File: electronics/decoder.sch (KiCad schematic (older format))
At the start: 8 parts, among them U33 AT28C64B, U40 AT28C64B, U41 AT28C64B, U44 AT28C64B

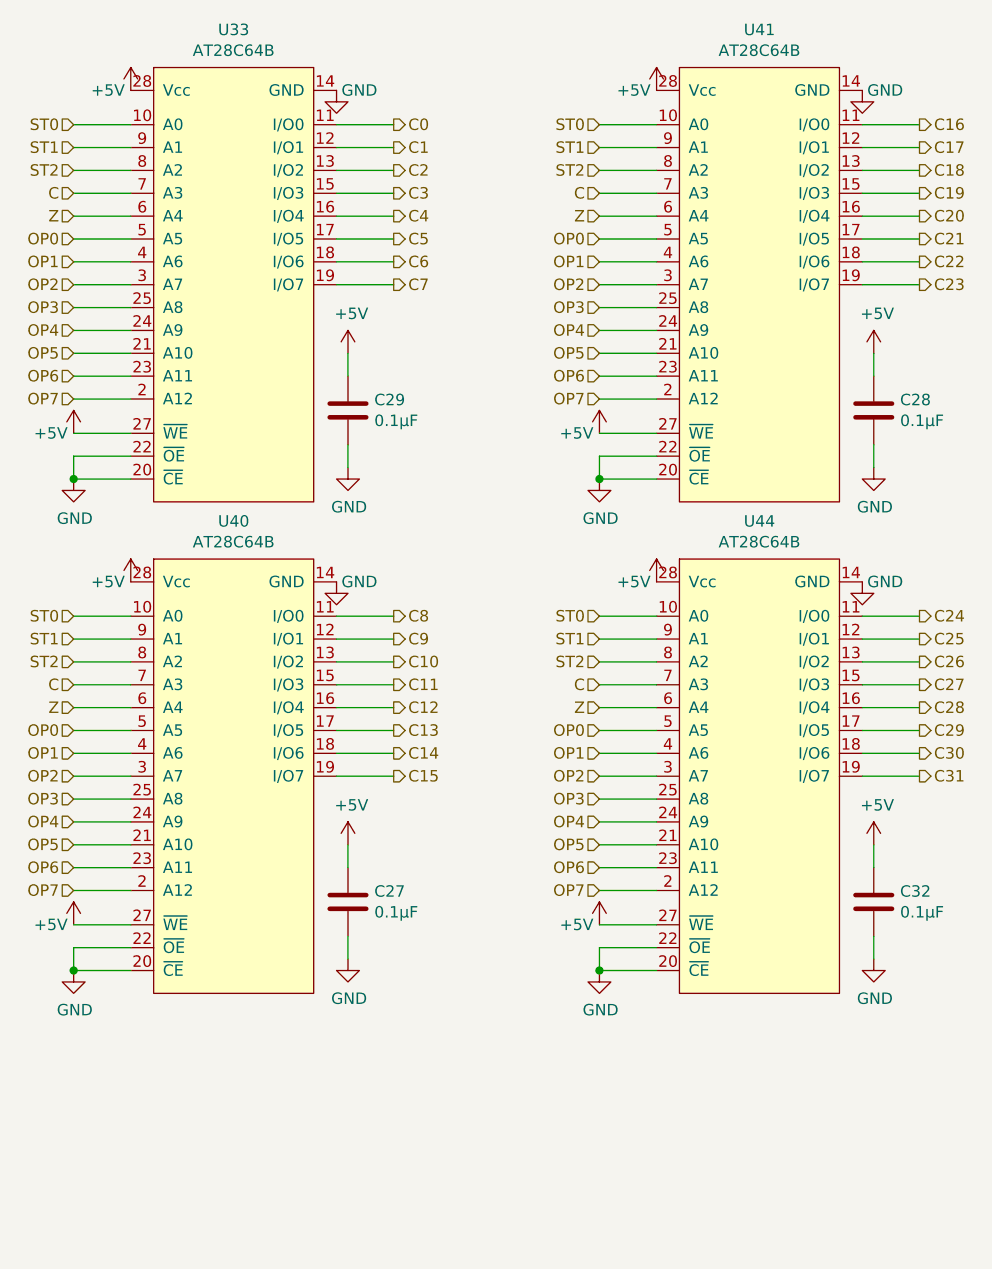
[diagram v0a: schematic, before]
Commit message: Some initial electronics design
Not everything done yet, just committing to show progress and to get the changes out of the way.
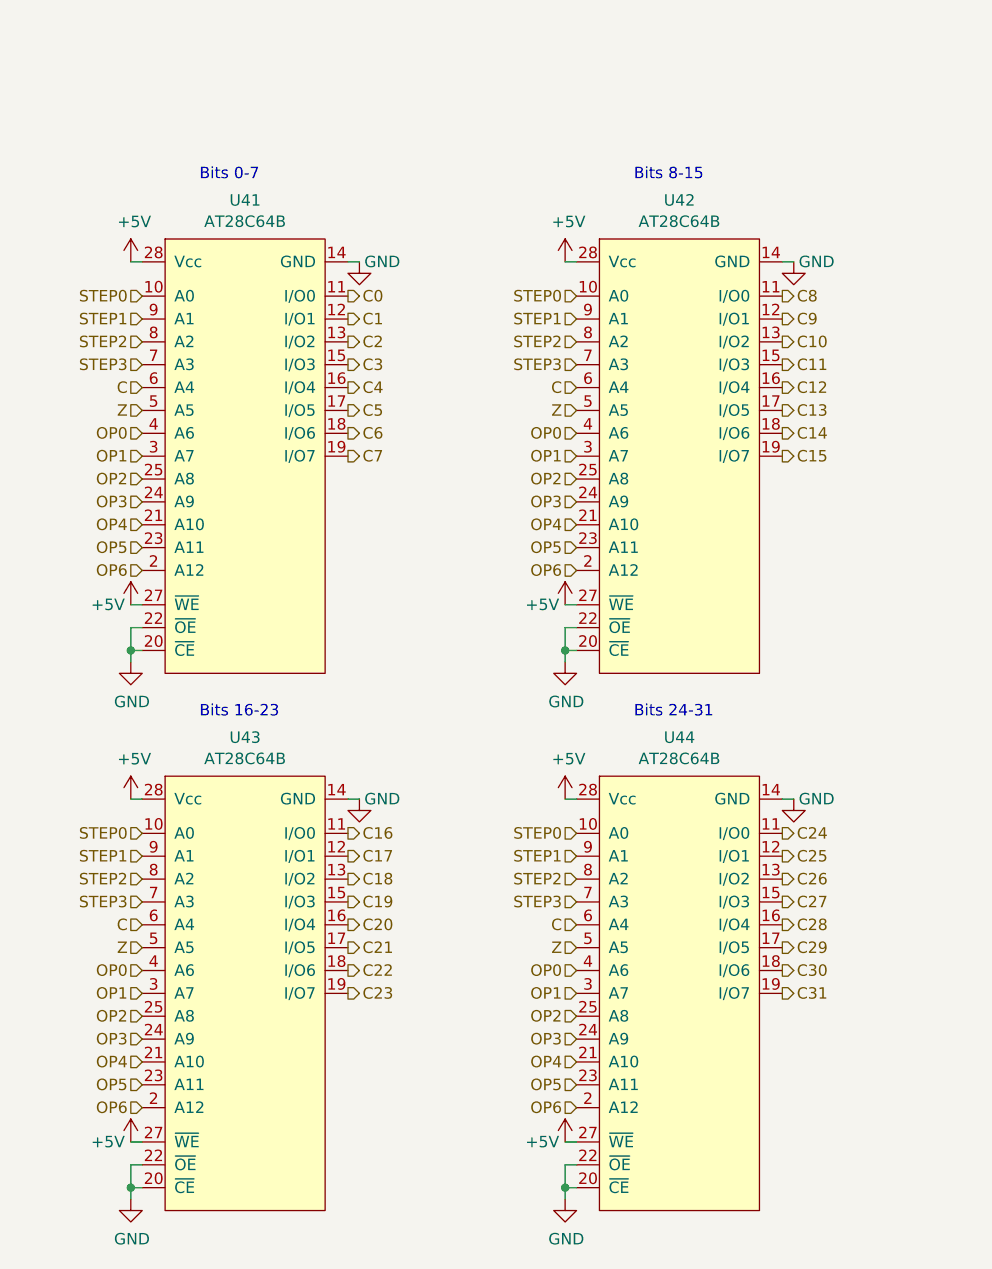
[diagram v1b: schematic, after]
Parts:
- removed C27, C28, C29, C32: 0.1µF, Capacitor_THT:CP_Radial_D4.0mm_P1.50mm, symbol Device:C
- removed U33, U40: AT28C64B, Package_DIP:AT28C64B, symbol misc_components:AT28C64B
- added U42, U43: AT28C64B, symbol misc_components:AT28C64B
- U41, U44: footprint Package_DIP:AT28C64B -> (none)
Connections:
- net OP7 is gone; now on net OP6: U41.2 (A12), U44.2 (A12)
- net +5V: now also U42.27 (~WE), U42.28 (Vcc), U43.27 (~WE), U43.28 (Vcc)
- net C: now also U41.6 (A4), U44.6 (A4), U42.6 (A4), U43.6 (A4); no longer U41.7 (A3), U44.7 (A3)
- net C0: now also U41.11 (I/O0)
- net C1: now also U41.12 (I/O1)
- net C10: now also U42.13 (I/O2)
- net C11: now also U42.15 (I/O3)
- net C12: now also U42.16 (I/O4)
- net C13: now also U42.17 (I/O5)
- net C14: now also U42.18 (I/O6)
- net C15: now also U42.19 (I/O7)
- net C16: now also U43.11 (I/O0); no longer U41.11 (I/O0)
- net C17: now also U43.12 (I/O1); no longer U41.12 (I/O1)
- net C18: now also U43.13 (I/O2); no longer U41.13 (I/O2)
- net C19: now also U43.15 (I/O3); no longer U41.15 (I/O3)
- net C2: now also U41.13 (I/O2)
- net C20: now also U43.16 (I/O4); no longer U41.16 (I/O4)
- net C21: now also U43.17 (I/O5); no longer U41.17 (I/O5)
- net C22: now also U43.18 (I/O6); no longer U41.18 (I/O6)
- net C23: now also U43.19 (I/O7); no longer U41.19 (I/O7)
- net C3: now also U41.15 (I/O3)
- net C4: now also U41.16 (I/O4)
- net C5: now also U41.17 (I/O5)
- net C6: now also U41.18 (I/O6)
- net C7: now also U41.19 (I/O7)
- net C8: now also U42.11 (I/O0)
- net C9: now also U42.12 (I/O1)
- net GND: now also U42.14 (GND), U42.20 (~CE), U42.22 (~OE), U43.14 (GND), U43.20 (~CE), U43.22 (~OE)
- net OP0: now also U41.4 (A6), U44.4 (A6), U42.4 (A6), U43.4 (A6); no longer U41.5 (A5), U44.5 (A5)
- net OP1: now also U41.3 (A7), U44.3 (A7), U42.3 (A7), U43.3 (A7); no longer U41.4 (A6), U44.4 (A6)
- net OP2: now also U41.25 (A8), U44.25 (A8), U42.25 (A8), U43.25 (A8); no longer U41.3 (A7), U44.3 (A7)
- net OP3: now also U41.24 (A9), U44.24 (A9), U42.24 (A9), U43.24 (A9); no longer U41.25 (A8), U44.25 (A8)
- net OP4: now also U41.21 (A10), U44.21 (A10), U42.21 (A10), U43.21 (A10); no longer U41.24 (A9), U44.24 (A9)
- net OP5: now also U41.23 (A11), U44.23 (A11), U42.23 (A11), U43.23 (A11); no longer U41.21 (A10), U44.21 (A10)
- net OP6: now also U42.2 (A12), U43.2 (A12); no longer U41.23 (A11), U44.23 (A11)
- net Z: now also U41.5 (A5), U44.5 (A5), U42.5 (A5), U43.5 (A5); no longer U41.6 (A4), U44.6 (A4)
- net ST0 renamed STEP0
- net STEP0: now also U42.10 (A0), U43.10 (A0)
- net ST1 renamed STEP1
- net STEP1: now also U42.9 (A1), U43.9 (A1)
- net ST2 renamed STEP2
- net STEP2: now also U42.8 (A2), U43.8 (A2)
- new net STEP3: U41.7 (A3), U42.7 (A3), U43.7 (A3), U44.7 (A3)
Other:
- note added: "Bits 0-7"
- note added: "Bits 16-23"
- note added: "Bits 24-31"
- note added: "Bits 8-15"
